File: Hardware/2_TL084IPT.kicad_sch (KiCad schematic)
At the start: 23 parts, among them J8 Screw_Terminal_01x08, Q4 N_Mosfet, Q5 N_Mosfet, Q6 N_Mosfet, Q7 N_Mosfet, U12 TL084

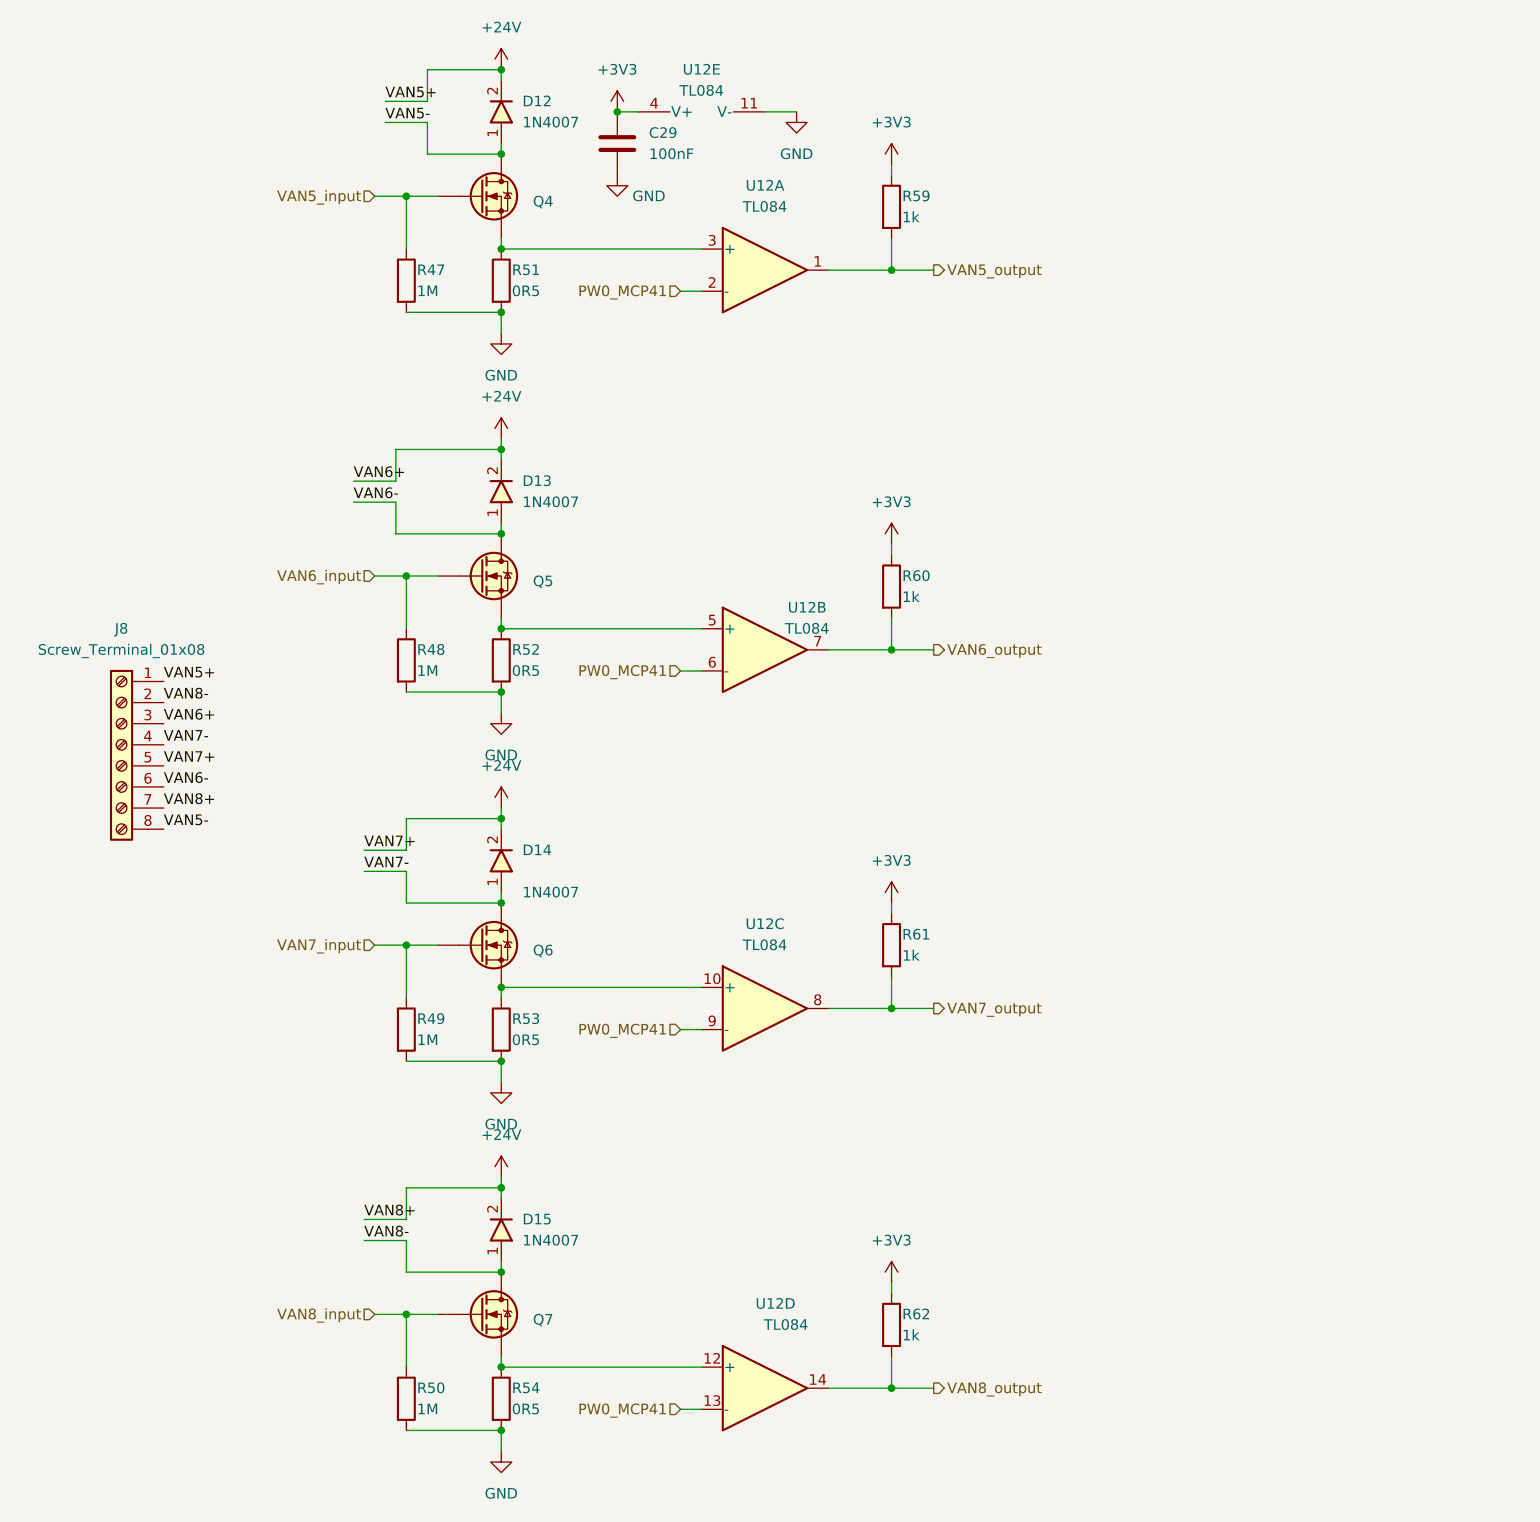
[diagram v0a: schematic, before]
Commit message: layout part 2
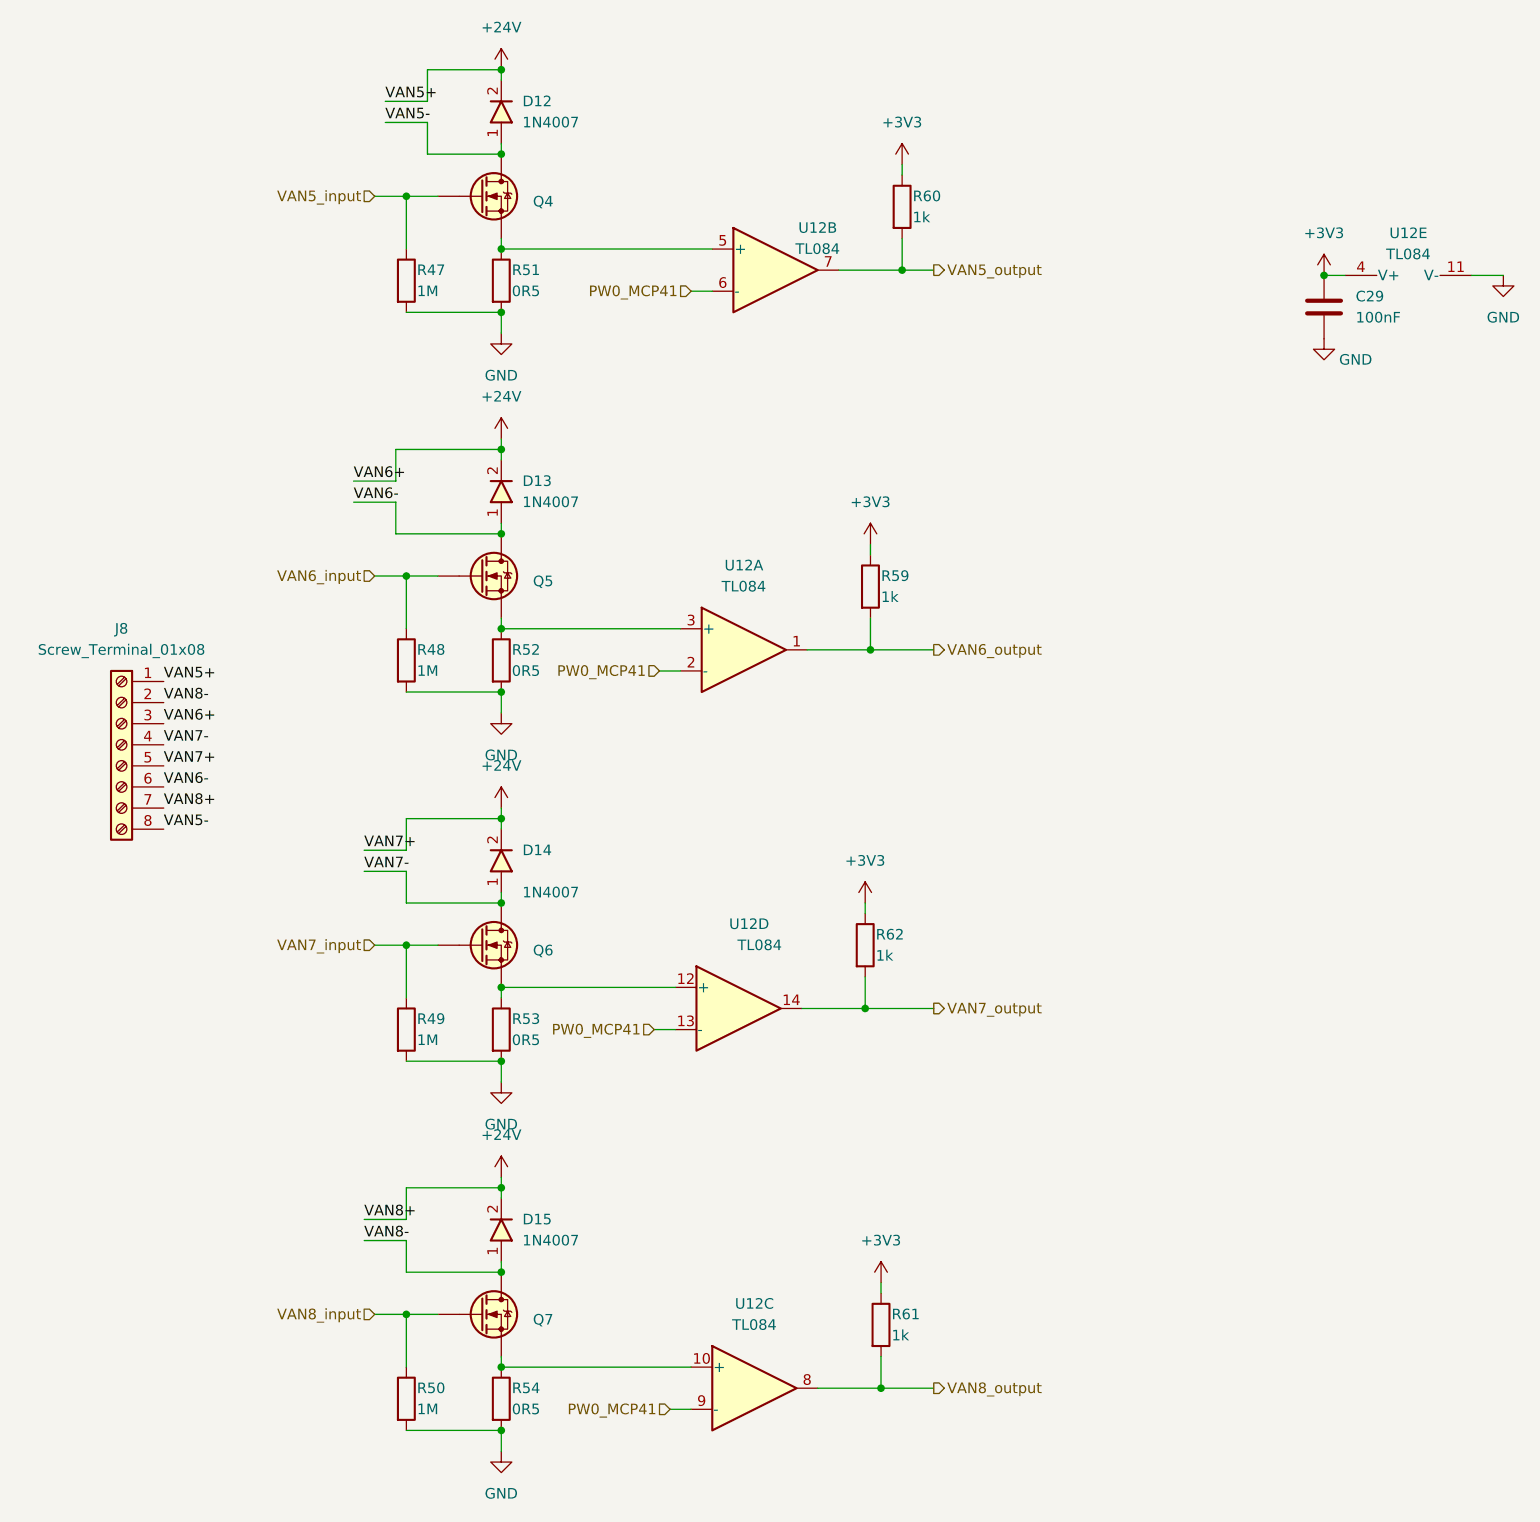
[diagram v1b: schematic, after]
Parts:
- D12, D13, D14, D15: footprint IVS_FOOTPRINTS:D_MiniMELF -> IVS_FOOTPRINTS:D_SOD323
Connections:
- net VAN5_output: now also R60.2, U12.7; no longer R59.2, U12.1
- net VAN6_output: now also R59.2, U12.1; no longer R60.2, U12.7
- net VAN7_output: now also R62.2, U12.14; no longer R61.2, U12.8
- net VAN8_output: now also R61.2, U12.8; no longer R62.2, U12.14
- net at Q4.2 (S), R51.1: now also U12.5 (+); no longer U12.3 (+)
- net at Q7.2 (S), R54.1: now also U12.10 (+); no longer U12.12 (+)
- net at Q5.2 (S), R52.1: now also U12.3 (+); no longer U12.5 (+)
- net at Q6.2 (S), R53.1: now also U12.12 (+); no longer U12.10 (+)
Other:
- moved on the sheet: C29, R59, R60, R61, R62, U12A, U12B, U12C, U12D, U12E
